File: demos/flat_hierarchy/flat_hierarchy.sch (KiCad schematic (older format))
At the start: 0 parts

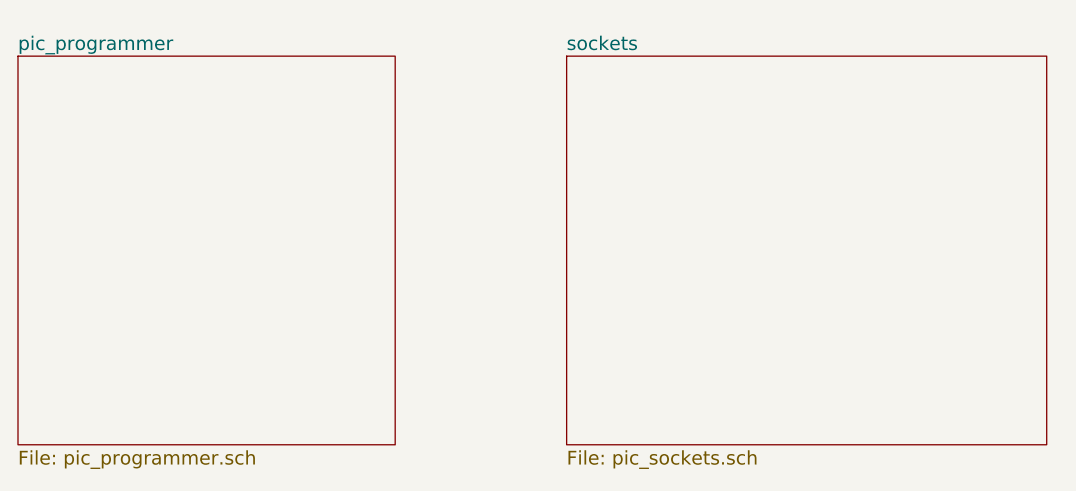
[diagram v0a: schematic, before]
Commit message: Imported Upstream version 4.0.0~rc1
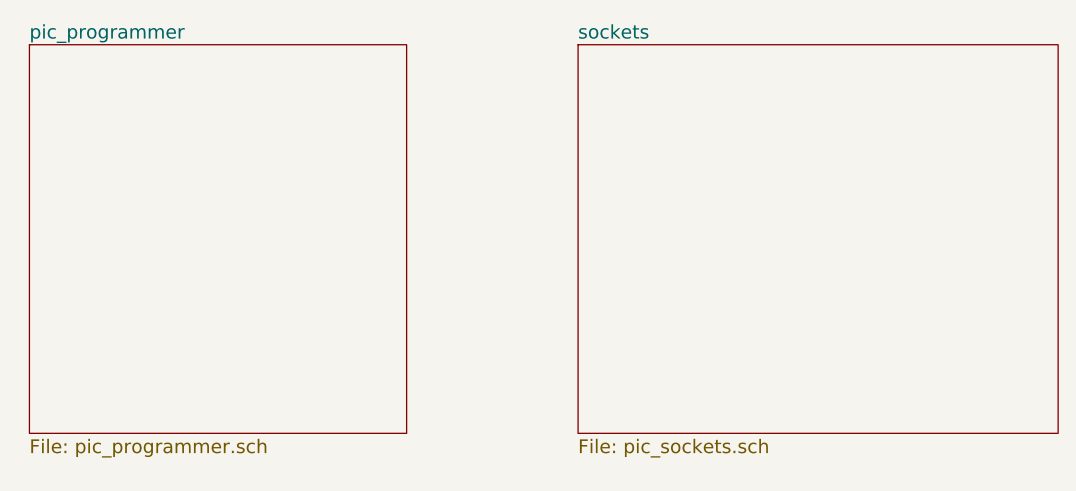
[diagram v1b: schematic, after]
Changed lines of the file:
@@
 EESchema Schematic File Version 2
-LIBS:power,device,transistors,conn,linear,regul,74xx,cmos4000,adc-dac,memory,xilinx,special,microcontrollers,dsp,microchip,analog_switches,motorola,texas,intel,audio,interface,digital-audio,philips,display,cypress,siliconi,contrib,valves
-EELAYER 23  0
+LIBS:flat_hierarchy_schlib
+LIBS:flat_hierarchy-cache
+EELAYER 25 0
 EELAYER END
-$Descr A4 11700 8267
+$Descr A4 11693 8268
+encoding utf-8
 Sheet 1 3
 Title ""
-Date "15 jun 2008"
+Date "Sun 22 Mar 2015"
 Rev "1"
 Comp ""
@@
 $EndDescr
 $Sheet
-S 5550 2650 2100 1700
+S 5600 2600 2100 1700
 U 48553E7C
 F0 "sockets" 60
@@
 $EndSheet
 $Sheet
-S 3150 2650 1650 1700
+S 3200 2600 1650 1700
 U 48553E53
 F0 "pic_programmer" 60
